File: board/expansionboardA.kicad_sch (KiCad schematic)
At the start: 66 parts, among them J1 USB_C_Receptacle, J2 USB_A_Stacked, J3 HDMI_A, J4 FAN, J5 DEBUG, U1 MAX3420EECJ, U2 GPIO_U2, U3 SII164CTG64, U4 GPIO_U4, U6 CS4344-CZZR, U7 MAX3421EEHJ+T, Y1 403C35D12M00000, Y2 403C35D12M00000

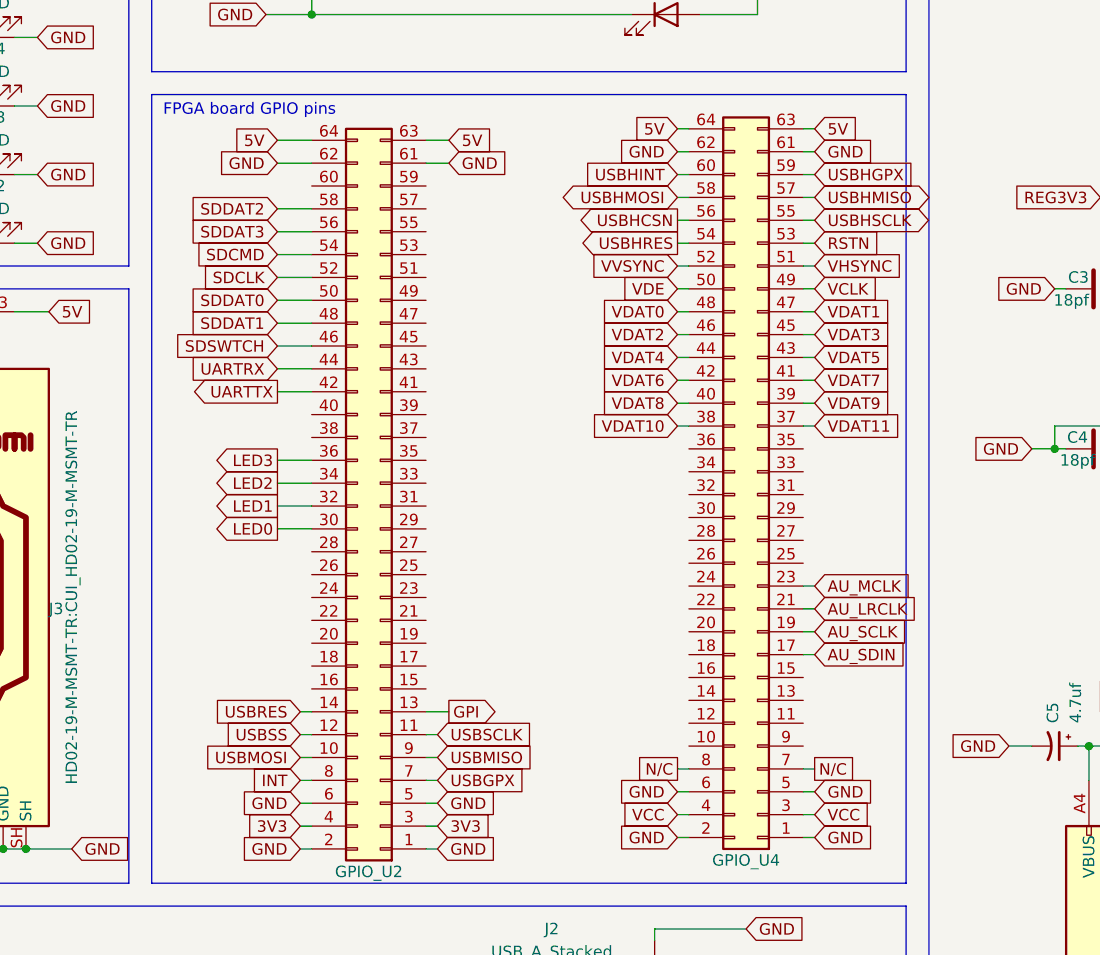
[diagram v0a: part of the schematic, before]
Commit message: Board and ROM updates
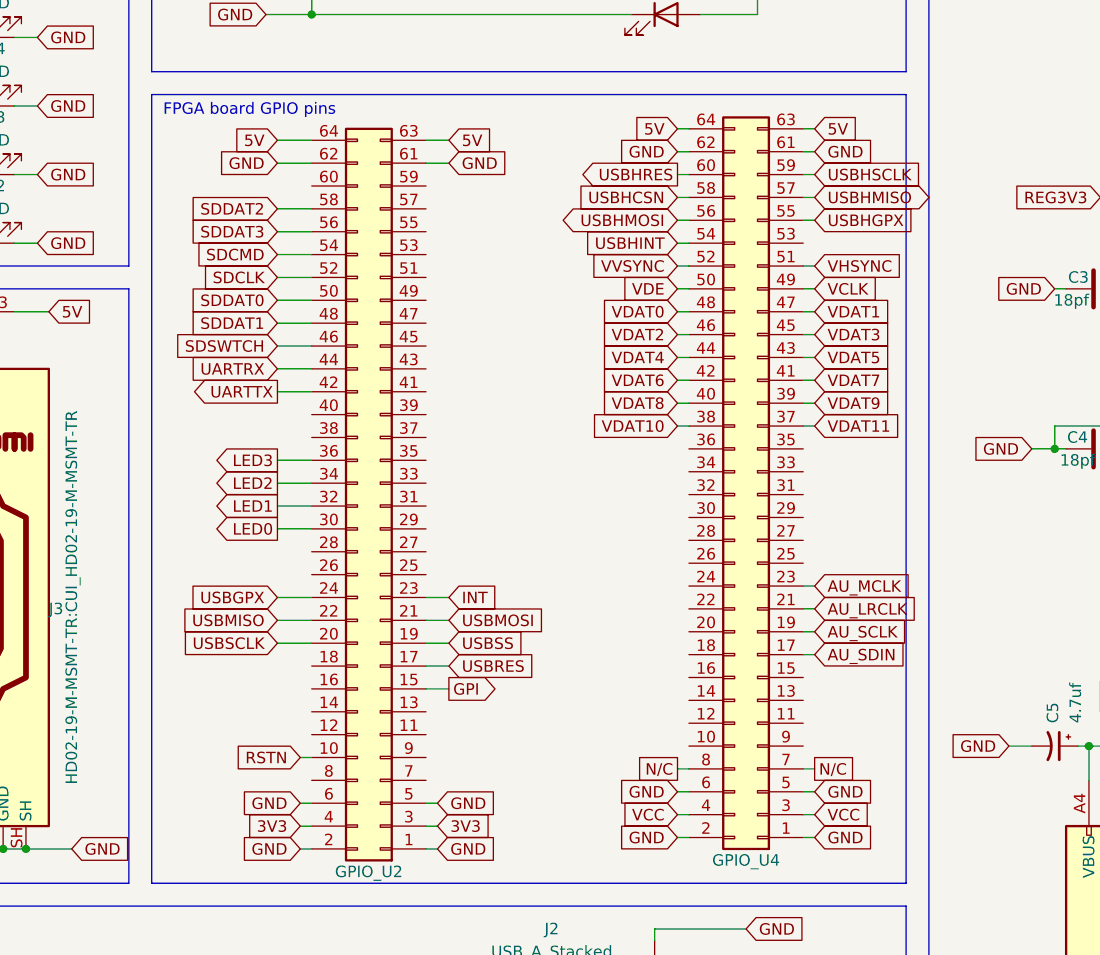
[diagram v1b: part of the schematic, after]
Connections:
- net GPI: now also U2.15 (Pin_15); no longer U2.13 (Pin_13)
- net INT: now also U2.23 (Pin_23); no longer U2.8 (Pin_8)
- net RSTN: now also U2.10 (Pin_10); no longer U4.53 (Pin_53)
- net USBGPX: now also U2.24 (Pin_24); no longer U2.7 (Pin_7)
- net USBHCSN: now also U4.58 (Pin_58); no longer U4.56 (Pin_56)
- net USBHGPX: now also U4.55 (Pin_55); no longer U4.59 (Pin_59)
- net USBHINT: now also U4.54 (Pin_54); no longer U4.60 (Pin_60)
- net USBHMOSI: now also U4.56 (Pin_56); no longer U4.58 (Pin_58)
- net USBHRES: now also U4.60 (Pin_60); no longer U4.54 (Pin_54)
- net USBHSCLK: now also U4.59 (Pin_59); no longer U4.55 (Pin_55)
- net USBMISO: now also U2.22 (Pin_22); no longer U2.9 (Pin_9)
- net USBMOSI: now also U2.21 (Pin_21); no longer U2.10 (Pin_10)
- net USBRES: now also U2.17 (Pin_17); no longer U2.14 (Pin_14)
- net USBSCLK: now also U2.20 (Pin_20); no longer U2.11 (Pin_11)
- net USBSS: now also U2.19 (Pin_19); no longer U2.12 (Pin_12)
